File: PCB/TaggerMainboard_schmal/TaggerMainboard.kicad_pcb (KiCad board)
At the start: 2 copper layers, 158 x 34 mm, 62 parts, among them J3 DFPlayer, J5 USB_OTG, Q1 FDN304P, SW1 SW_Reset, U1 MCU-ATMEGA2560-16AU(TQFP100), U2 IRLML2502, U3 LM2596S-5, U4 LMV358, U5 AMS1117-3.3, U6 FT232RL, Y1 CSTCE16M0V53-R0

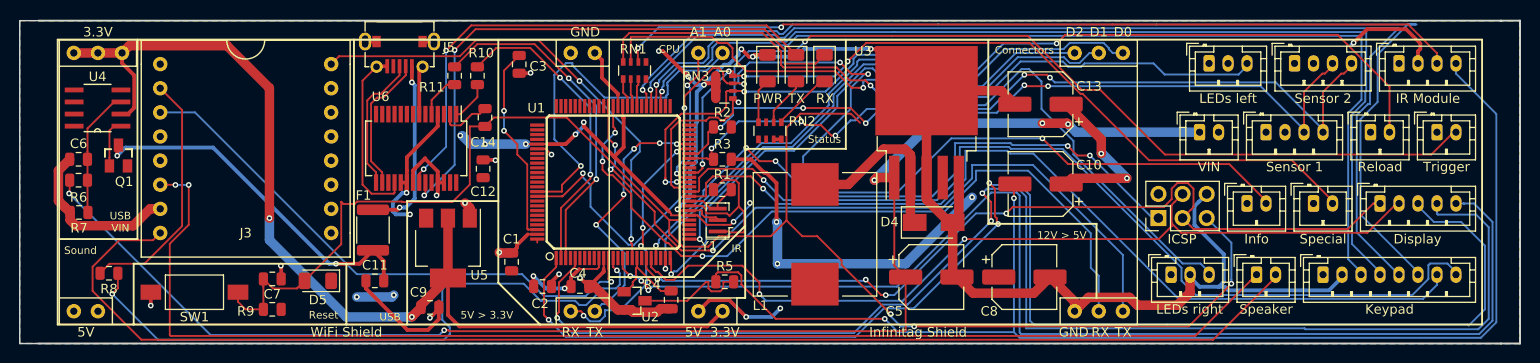
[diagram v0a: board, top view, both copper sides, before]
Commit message: Updates
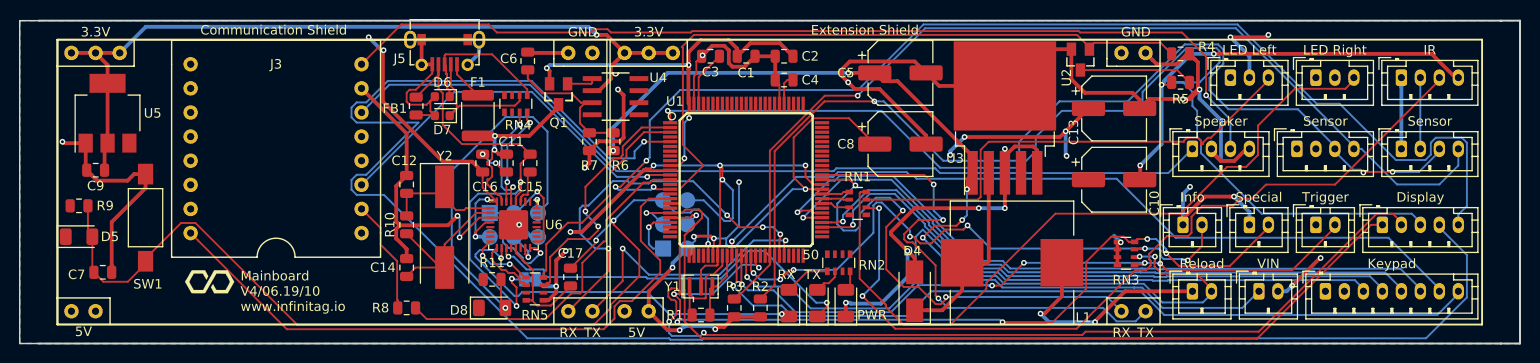
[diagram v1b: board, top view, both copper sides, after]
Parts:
- removed ICSP: ICSP, Connector_PinHeader_2.54mm:PinHeader_2x03_P2.54mm_Vertical
- removed IR Module: JST_PH_IrLED, Connector_JST:JST_PH_B4B-PH-K_1x04_P2.00mm_Vertical
- removed Infinitag Shield: Infinitag_Shield_lang, Infinitag:Infinitag_Shield_lang
- removed LEDs left: JST_PH_LEDbar_left, Connector_JST:JST_PH_B3B-PH-K_1x03_P2.00mm_Vertical
- removed LEDs right: JST_PH_LEDbar_right, Connector_JST:JST_PH_B3B-PH-K_1x03_P2.00mm_Vertical
- removed Sensor 1: JSP_PH_Sensor, Connector_JST:JST_PH_B4B-PH-K_1x04_P2.00mm_Vertical
- removed Sensor 2: JSP_PH_Sensor, Connector_JST:JST_PH_B4B-PH-K_1x04_P2.00mm_Vertical
- removed the Speaker at (160.2, 44.8)
- removed WiFi Shield: WiFi Connector, Infinitag:Infinitag_ESP_Shield_Lang
- added C15: 1u, Capacitor_SMD:C_0805_2012Metric, F.Cu at (83.8, 33.0)
- added C16: 100n, Capacitor_SMD:C_0805_2012Metric, F.Cu at (78.8, 33.0)
- added C17: 100nF, Capacitor_SMD:C_0805_2012Metric, F.Cu at (88.0, 45.0)
- added Communication Shield: WiFi Connector, Infinitag:Infinitag_ESP_Shield_Lang, F.Cu at (134.0, 50.0)
- added D6: CG0603MLC-05E, Diode_SMD:D_0603_1608Metric, F.Cu at (74.5, 26.0)
- added D7: CG0603MLC-05E, Diode_SMD:D_0603_1608Metric, F.Cu at (74.5, 28.0)
- added D8: CD1206-S01575, Diode_SMD:D_1206_3216Metric, F.Cu at (79.8, 48.2)
- added Extension Shield: Infinitag_ESP_Shield_Lang, Infinitag:Infinitag_ESP_Shield_Lang, F.Cu at (192.2, 50.0)
- added FB1: BLM21PG 221, Inductor_SMD:L_0805_2012Metric, F.Cu at (71.8, 27.0)
- added G***: Bildmarke_6x6mm, Infinitag:Bildmarke_6x6mm, F.Cu at (50.0, 45.5)
- added IR: JST_PH_IrLED, Connector_JST:JST_PH_B4B-PH-K_1x04_P2.00mm_Vertical, F.Cu at (175.5, 24.0)
- added J19: Conn_02x03_Odd_Even, Infinitag:ICSP_Pogo, B.Cu at (79.5, 38.2)
- added J6: ICSP, Infinitag:ICSP_Pogo, B.Cu at (97.8, 42.0)
- added JP1: SolderJumper_2_Bridged, Jumper:SolderJumper-2_P1.3mm_Bridged_Pad1.0x1.5mm, B.Cu at (83.8, 45.2)
- added LED Left: JST_PH_LEDbar_left, Connector_JST:JST_PH_B3B-PH-K_1x03_P2.00mm_Vertical, F.Cu at (157.5, 24.0)
- added LED Right: JST_PH_LEDbar_right, Connector_JST:JST_PH_B3B-PH-K_1x03_P2.00mm_Vertical, F.Cu at (166.5, 24.0)
- added RN4: 22R, Resistor_SMD:R_Array_Convex_4x0603, F.Cu at (82.2, 26.8)
- added RN5: 1K, Resistor_SMD:R_Array_Convex_4x0603, F.Cu at (84.2, 46.2)
- added Sensor: JSP_PH_Sensor, Connector_JST:JST_PH_B4B-PH-K_1x04_P2.00mm_Vertical, F.Cu at (164.5, 31.5)
- added Sensor: JSP_PH_Sensor, Connector_JST:JST_PH_B4B-PH-K_1x04_P2.00mm_Vertical, F.Cu at (175.5, 31.5)
- added Speaker: JST_PH_Speaker, Connector_JST:JST_PH_B4B-PH-K_1x04_P2.00mm_Vertical, F.Cu at (153.5, 31.5)
- added Y2: 16MHz, Crystal:Crystal_SMD_HC49-SD, F.Cu at (74.8, 39.8)
- C11: value 100nF -> 100n
- C12, C14: value 100nF -> 22p
- R10: value 1K -> 1M
- R11: value 1K -> 10K
- U6: value FT232RL -> ATmega16U2-MU; footprint Package_SO:SSOP-28_5.3x10.2mm_P0.65mm -> Package_DFN_QFN:QFN-32-1EP_5x5mm_P0.5mm_EP3.1x3.1mm
- moved R4 59.6 mm to (152.2, 21.5), turned to 0 degrees
- moved R6 56.4 mm to (92.5, 30.8), turned to 90 degrees
- moved U4 54.6 mm to (92.8, 26.0), turned to 0 degrees
- moved R7 54.3 mm to (90.0, 30.8), turned to 270 degrees
- moved U2 53.4 mm to (141.7, 22.1), turned to 180 degrees
- moved R5 52.4 mm to (152.2, 24.5)
- moved C6 48.4 mm to (83.5, 22.2), turned to 90 degrees
- moved Q1 46.8 mm to (86.8, 25.8), turned to 180 degrees
- moved RN3 45.8 mm to (146.5, 42.5)
- moved U5 38.6 mm to (39.2, 27.8), turned to 90 degrees
- moved C9 38.1 mm to (38.0, 33.8), turned to 180 degrees
- moved C2 35.1 mm to (110.5, 21.8), turned to 180 degrees
- moved C1 32.8 mm to (106.5, 21.8), turned to 0 degrees
- moved R8 31.6 mm to (70.8, 48.2)
- moved C4 30.6 mm to (110.5, 24.2), turned to 180 degrees
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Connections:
- C12 pad 1: +5V -> Net-(C12-Pad1)
- C14 pad 2: RESET -> GND
- J3 pad 6: DF_SPK+ -> DF_SPK_LEFT
- J3 pad 8: DF_SPK- -> DF_SPK_RIGHT
- J5 pad 2: Net-(J5-Pad2) -> Net-(D7-Pad1)
- J5 pad 3: Net-(J5-Pad3) -> Net-(D6-Pad1)
- J5 pad 4: (no net) -> Net-(C15-Pad2)
- J5 pad 5: GND -> Net-(D6-Pad2)
- J5 pad 6: GND -> Net-(D6-Pad2)
- R10 pad 1: RX0 -> Net-(C12-Pad1)
- R10 pad 2: Net-(R10-Pad2) -> Net-(C14-Pad1)
- R11 pad 1: Net-(R11-Pad1) -> Net-(D8-Pad2)
- R11 pad 2: TX0 -> +5V
- U6 pad 1: Net-(R10-Pad2) -> Net-(C12-Pad1)
- U6 pad 10: (no net) -> LED_RX
- U6 pad 11: (no net) -> LED_TX
- U6 pad 13: (no net) -> Net-(C17-Pad2)
- U6 pad 15: Net-(J5-Pad3) -> Net-(J19-Pad4)
- U6 pad 16: Net-(J5-Pad2) -> Net-(J19-Pad1)
- U6 pad 17: (no net) -> Net-(J19-Pad3)
- U6 pad 18: GND -> (no net)
- U6 pad 19: +5V -> (no net)
- U6 pad 20: +5V -> (no net)
- U6 pad 21: GND -> (no net)
- U6 pad 22: LED_TX -> (no net)
- U6 pad 23: LED_RX -> (no net)
- U6 pad 24: (no net) -> Net-(D8-Pad2)
- U6 pad 25: GND -> (no net)
- U6 pad 26: GND -> (no net)
- U6 pad 27: (no net) -> Net-(C15-Pad1)
- U6 pad 28: (no net) -> Net-(C15-Pad2)
- U6 pad 3: (no net) -> GND
- U6 pad 5: Net-(R11-Pad1) -> (no net)
- U6 pad 7: GND -> (no net)
- U6 pad 8: (no net) -> Net-(RN5-Pad1)
- U6 pad 9: (no net) -> Net-(RN5-Pad2)
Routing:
- net DF_SPK-: track 140.8 -> 0.00 mm
- net DF_SPK+: track 136.8 -> 0.00 mm, vias 2 -> 0
- net DF_SPK_RIGHT: track 0.00 -> 103.3 mm, vias 0 -> 1
- net DF_SPK_LEFT: track 0.00 -> 93.9 mm
- net IR_LED_GND: track 131.8 -> 45.8 mm, vias 2 -> 3
- net +5V: track 147.3 -> 215.9 mm, vias 20 -> 23
- net IR_LED_SEND: track 8.87 -> 73.0 mm
- net Shield_D0: track 64.0 -> 0.00 mm, vias 1 -> 0
- net MISO: track 68.5 -> 5.94 mm, vias 5 -> 1
- net RESET: track 166.8 -> 104.4 mm
- net Shield_D1: track 61.8 -> 0.00 mm, vias 1 -> 0
- net GND: track 271.0 -> 329.9 mm, vias 19 -> 29
- net VIN_on: track 152.1 -> 97.6 mm
- net Shield_D2: track 53.2 -> 0.00 mm, vias 1 -> 0
- net Net-(C15-Pad2): track 0.00 -> 51.1 mm, vias 0 -> 3
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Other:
- board text added: "Mainboard V4/06.19/10 www.infinitag.io"
- board text removed: "12V > 5V"
- board text removed: "5V > 3.3V"
- board text removed: "CPU"
- board text removed: "Connectors"
- board text removed: "IR"
- board text removed: "Reset"
- board text removed: "Sound"
- board text removed: "Status"
- board text removed: "USB"
- board text removed: "USB VIN"
